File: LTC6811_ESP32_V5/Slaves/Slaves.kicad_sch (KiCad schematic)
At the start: 43 parts, among them J22 B2P-VH-B, J6 B2P-VH-B, J9 B2P-VH-B

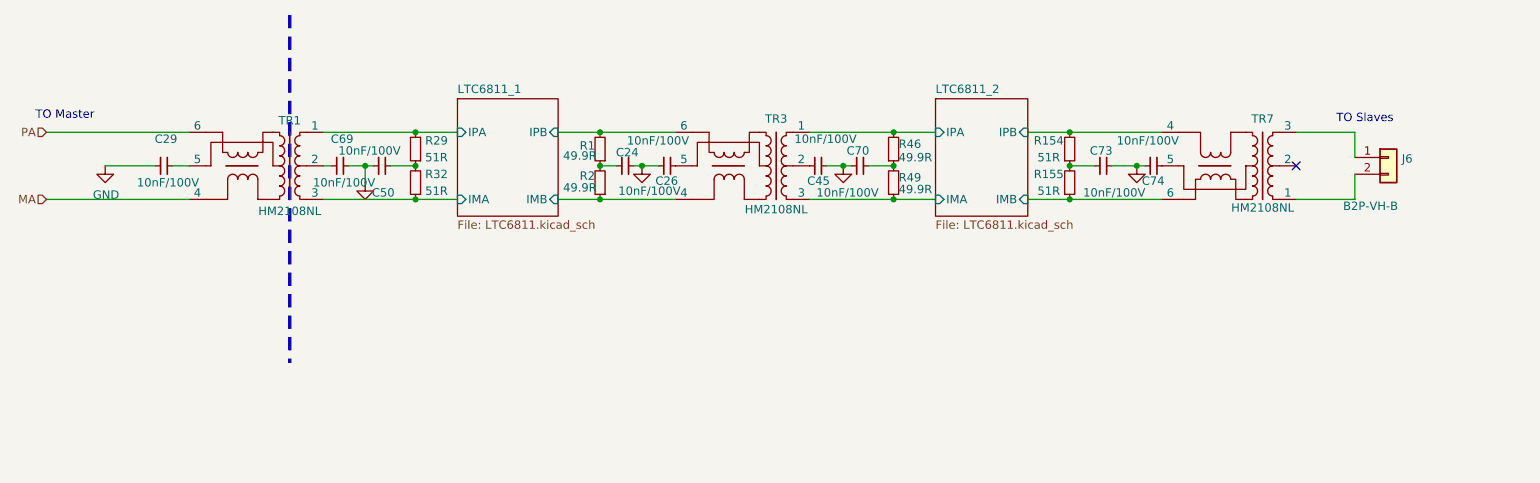
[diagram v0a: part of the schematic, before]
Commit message: Add files via upload
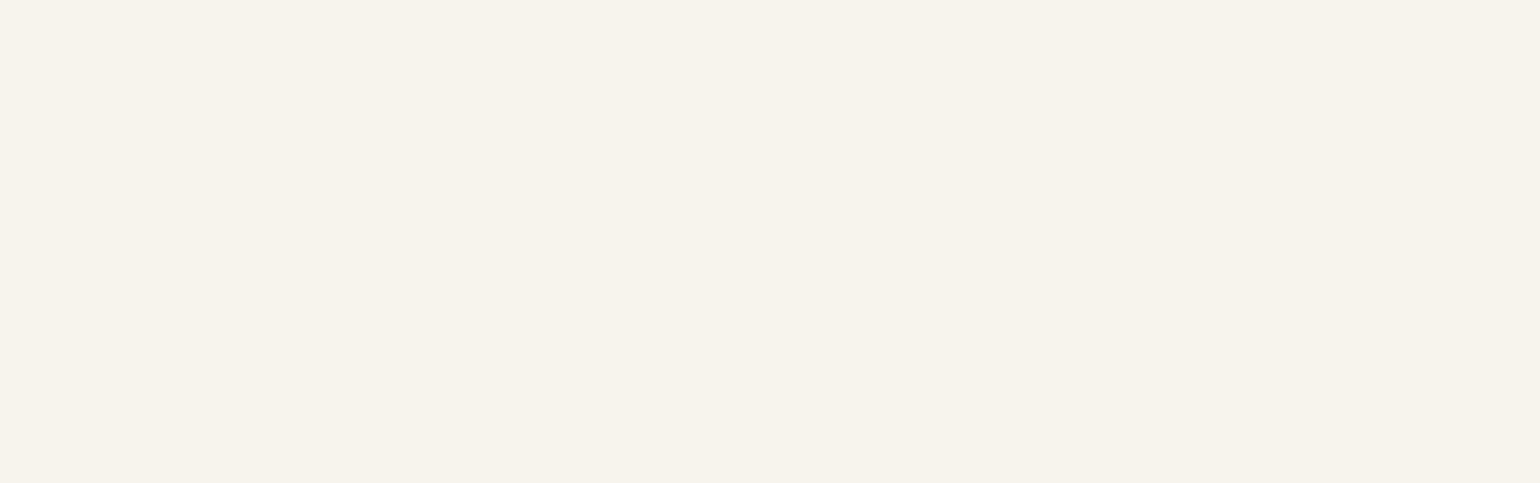
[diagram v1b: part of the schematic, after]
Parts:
- removed C24, C26, C29, C45, C50, C69, C70, C73, C74: 10nF/100V, Capacitor_SMD:C_0603_1608Metric, symbol Library:C
- removed J6: B2P-VH-B, Connector_JST:JST_VH_B2P-VH-B_1x02_P3.96mm_Vertical, symbol Library:Conn_01x02
- removed R1, R2, R46, R49: 49.9R, Resistor_SMD:R_0603_1608Metric, symbol Library:R_Small
- removed R154, R155, R29, R32: 51R, Resistor_SMD:R_0603_1608Metric, symbol Library:R_Small
- removed TR1, TR3, TR7: HM2108NL, Transformer_SMD:HM2108NL, symbol Library:HM2108NL
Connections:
- no-connect marks 3 -> 2
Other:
- removed sheet LTC6811_1
- removed sheet LTC6811_2
- note removed: "TO Master"
